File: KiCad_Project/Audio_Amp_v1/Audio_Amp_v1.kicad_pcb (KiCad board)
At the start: 2 copper layers, 93.5 x 52.8 mm, 61 parts, among them IC2 TPA3116D2DAD, IC4 LMR33630ADDA, J1 TS-103-T-A, J2 1729128, J3 1729128, J4 PJ-102AH

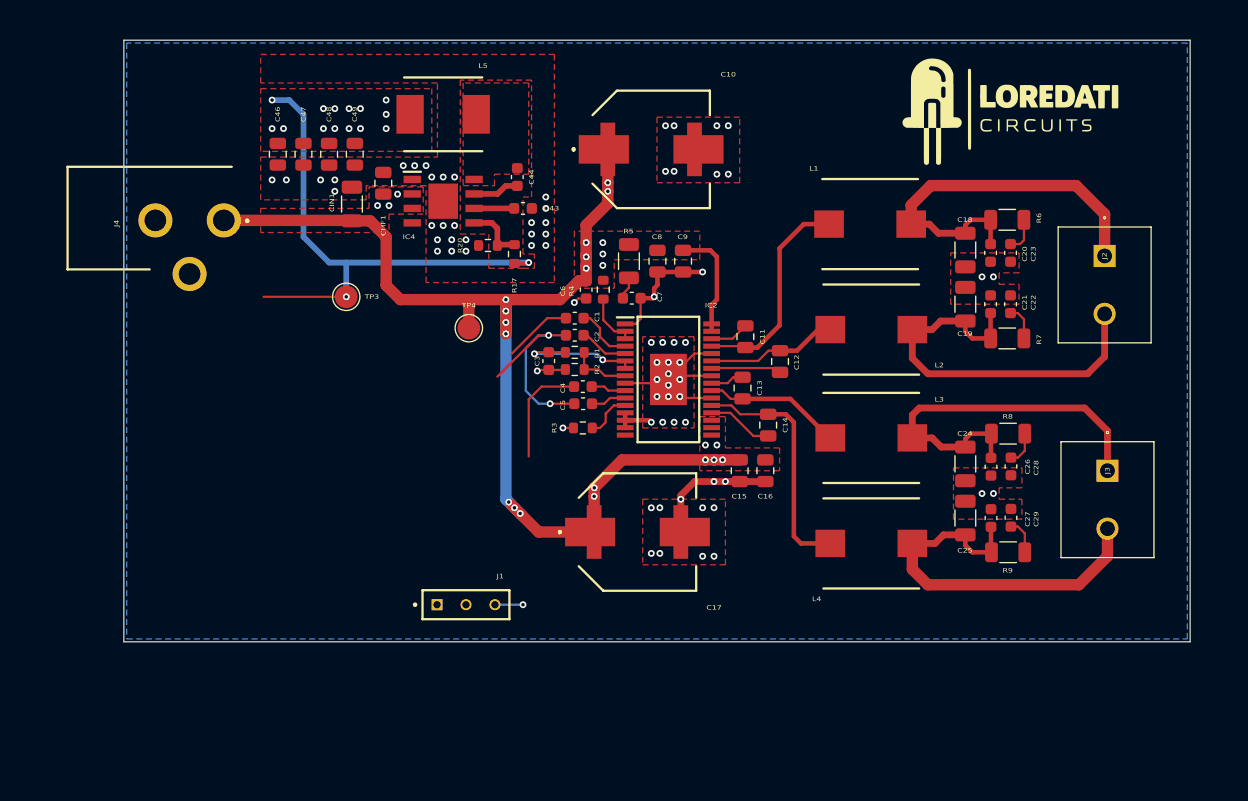
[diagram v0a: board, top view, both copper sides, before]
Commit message: Started routing
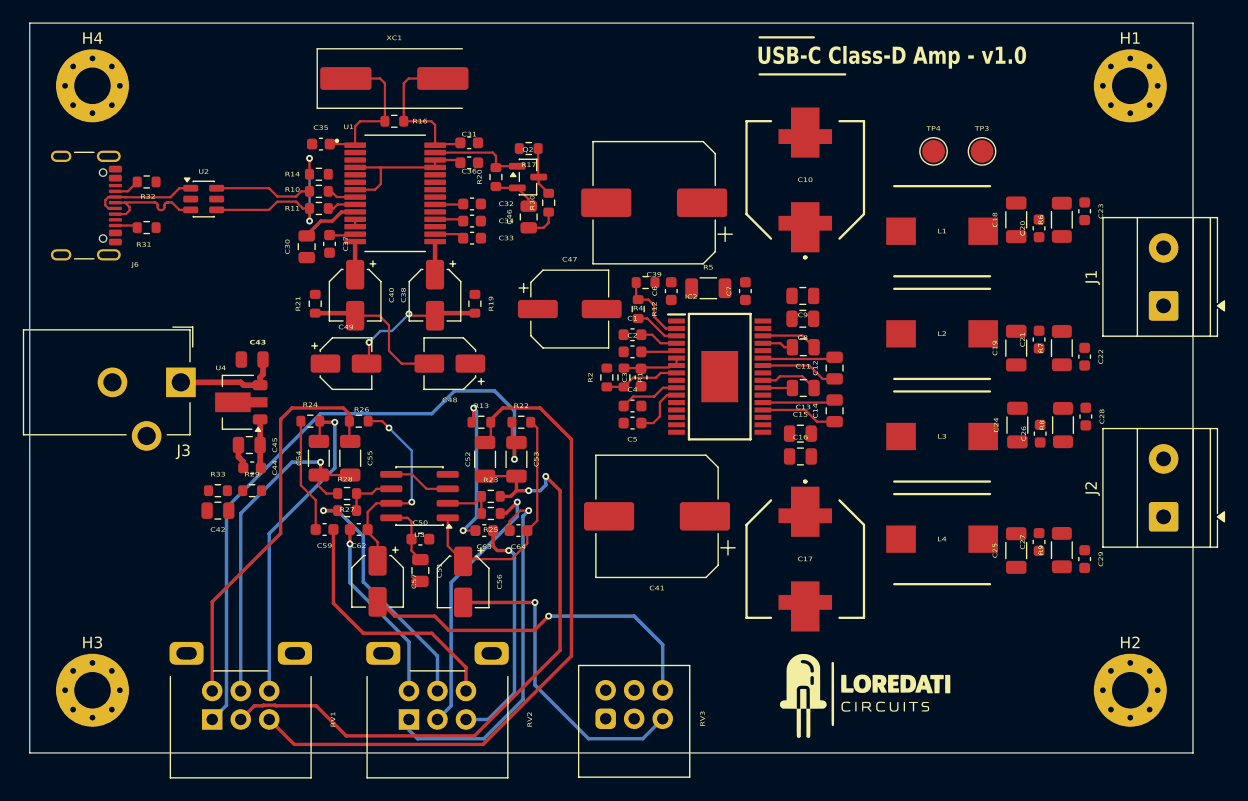
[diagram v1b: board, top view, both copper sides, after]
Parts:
- removed CHF1: 220n, Capacitor_SMD:C_0805_2012Metric
- removed CIN1: 10u, Capacitor_SMD:C_1206_3216Metric
- removed IC4: LMR33630ADDA, LMR33630:SOIC127P600X170-9N
- removed J4: PJ-102AH, 24V-JACK:PJ-102AH
- removed L5: IHLP2525CZER6R8M8A, IHLP2525CZER6R8M8A:INDPM6965X300N
- removed R3: 100k, Resistor_SMD:R_0603_1608Metric
- added C30: 10u, Capacitor_SMD:C_0805_2012Metric, F.Cu at (86.8, 96.9)
- added C31: 1u, Capacitor_SMD:C_0603_1608Metric, F.Cu at (101.0, 89.5)
- added C32: 1u, Capacitor_SMD:C_0603_1608Metric, F.Cu at (101.3, 93.1)
- added C33: 1u, Capacitor_SMD:C_0603_1608Metric, F.Cu at (101.3, 96.1)
- added C34: 10u, Capacitor_SMD:C_0603_1608Metric, F.Cu at (101.3, 94.6)
- added C35: 33p, Capacitor_SMD:C_0603_1608Metric, F.Cu at (88.0, 87.9)
- added C36: 33p, Capacitor_SMD:C_0603_1608Metric, F.Cu at (101.0, 87.8)
- added C37: 1u, Capacitor_SMD:C_0603_1608Metric, F.Cu at (88.8, 96.6)
- added C38: 10u, Capacitor_SMD:CP_Elec_4x5.8, F.Cu at (98.0, 101.1)
- added C39: 470u, Capacitor_SMD:CP_Elec_10x10.5, F.Cu at (117.2, 93.0)
- added C40: 10u, Capacitor_SMD:CP_Elec_4x5.8, F.Cu at (91.0, 101.1)
- added C41: 470u, Capacitor_SMD:CP_Elec_10x10.5, F.Cu at (117.5, 120.5)
- added C42: 10u, Capacitor_SMD:C_0805_2012Metric, F.Cu at (79.0, 120.0)
- added C45: 10u, Capacitor_SMD:C_0805_2012Metric, F.Cu at (81.8, 114.2)
- added C50: 100n, Capacitor_SMD:C_0603_1608Metric, F.Cu at (96.8, 122.5)
- added C51: 10u, Capacitor_SMD:C_0805_2012Metric, F.Cu at (96.8, 125.2)
- added C52: 100n, Capacitor_SMD:C_1206_3216Metric, F.Cu at (102.4, 115.5)
- added C53: 100n, Capacitor_SMD:C_1206_3216Metric, F.Cu at (105.2, 115.5)
- added C54: 100n, Capacitor_SMD:C_1206_3216Metric, F.Cu at (87.8, 115.4)
- added C55: 100n, Capacitor_SMD:C_1206_3216Metric, F.Cu at (90.6, 115.4)
- added C56: 10u, Capacitor_SMD:CP_Elec_4x5.8, F.Cu at (100.5, 126.2)
- added C57: 10u, Capacitor_SMD:CP_Elec_4x5.8, F.Cu at (93.0, 126.2)
- added C59: 2n2, Capacitor_SMD:C_0603_1608Metric, F.Cu at (88.3, 121.7)
- added C62: 2n2, Capacitor_SMD:C_0603_1608Metric, F.Cu at (91.3, 121.7)
- added C63: 2n2, Capacitor_SMD:C_0603_1608Metric, F.Cu at (102.3, 121.8)
- added C64: 2n2, Capacitor_SMD:C_0603_1608Metric, F.Cu at (105.3, 121.8)
- added H1: MountingHole_Pad, MountingHole:MountingHole_3.2mm_M3_Pad_Via, F.Cu at (159.0, 82.8)
- added H2: MountingHole_Pad, MountingHole:MountingHole_3.2mm_M3_Pad_Via, F.Cu at (159.0, 135.8)
- added H3: MountingHole_Pad, MountingHole:MountingHole_3.2mm_M3_Pad_Via, F.Cu at (68.0, 135.8)
- added H4: MountingHole_Pad, MountingHole:MountingHole_3.2mm_M3_Pad_Via, F.Cu at (68.0, 82.8)
- added J6: USB_C_Receptacle_USB2.0_16P, Connector_USB:USB_C_Receptacle_GCT_USB4105-xx-A_16P_TopMnt_Horizontal, F.Cu at (66.3, 93.2)
- added Q2: BSS138, Package_TO_SOT_SMD:SOT-23, F.Cu at (106.2, 90.8)
- added R10: 22, Resistor_SMD:R_0603_1608Metric, F.Cu at (87.9, 92.0)
- added R11: 22, Resistor_SMD:R_0603_1608Metric, F.Cu at (87.9, 93.5)
- added R12: 1k, Resistor_SMD:R_0603_1608Metric, F.Cu at (115.8, 102.3)
- added R13: 10k, Resistor_SMD:R_0603_1608Metric, F.Cu at (102.1, 112.2)
- added R14: 1.5k, Resistor_SMD:R_0603_1608Metric, F.Cu at (87.9, 90.5)
- added R16: 1M, Resistor_SMD:R_0603_1608Metric, F.Cu at (94.5, 85.9)
- added R19: 47k, Resistor_SMD:R_0603_1608Metric, F.Cu at (101.5, 101.9)
- added R21: 47k, Resistor_SMD:R_0603_1608Metric, F.Cu at (87.5, 101.9)
- added R22: 10k, Resistor_SMD:R_0603_1608Metric, F.Cu at (105.6, 112.2)
- added R23: 10k, Resistor_SMD:R_0603_1608Metric, F.Cu at (102.9, 118.8)
- added R24: 10k, Resistor_SMD:R_0603_1608Metric, F.Cu at (87.1, 112.2)
- added R25: 3k3, Resistor_SMD:R_0603_1608Metric, F.Cu at (102.9, 120.2)
- added R26: 10k, Resistor_SMD:R_0603_1608Metric, F.Cu at (91.3, 112.2)
- added R27: 10k, Resistor_SMD:R_0603_1608Metric, F.Cu at (90.3, 118.5)
- added R28: 3k3, Resistor_SMD:R_0603_1608Metric, F.Cu at (90.3, 120.0)
- added R29: 100k, Resistor_SMD:R_0603_1608Metric, F.Cu at (82.0, 118.2)
- added R30: 100k, Resistor_SMD:R_0603_1608Metric, F.Cu at (108.0, 93.0)
- added R31: 5k1, Resistor_SMD:R_0603_1608Metric, F.Cu at (72.8, 95.2)
- added R32: 5k1, Resistor_SMD:R_0603_1608Metric, F.Cu at (72.8, 91.2)
- added R33: 100k, Resistor_SMD:R_0603_1608Metric, F.Cu at (79.0, 118.2)
- added RV1: 100k, Potentiometer_THT:Potentiometer_Alps_RK09L_Double_Horizontal, F.Cu at (78.5, 138.3)
- added RV2: 100k, Potentiometer_THT:Potentiometer_Alps_RK09L_Double_Horizontal, F.Cu at (95.8, 138.3)
- added RV3: 10k, Potentiometer_THT:Potentiometer_Alps_RK097_Dual_Horizontal, F.Cu at (113.0, 138.2)
- added U1: PCM2704CDB, PCM2704CDB:SOP65P780X200-28N, F.Cu at (94.5, 92.2)
- added U2: USBLC6-2SC6, Package_TO_SOT_SMD:SOT-23-6, F.Cu at (77.8, 92.7)
- added U3: OPA1678IDR, Package_SO:SOIC-8_3.9x4.9mm_P1.27mm, F.Cu at (96.7, 118.7)
- added U4: L78L12_SOT89, Package_TO_SOT_SMD:SOT-89-3, F.Cu at (80.8, 110.5)
- added XC1: 12Mhz, Crystal:Crystal_SMD_HC49-SD, F.Cu at (94.5, 82.1)
- C1, C2, C4, C5: value 1u -> 3u3
- C43: value 1u -> 0.33u; footprint Capacitor_SMD:C_0603_1608Metric -> PCM_JLCPCB:C_0805
- C44: value 100n -> 0.1u
- C46: value 22u -> 4u7
- C47: value 22u -> 47u; footprint Capacitor_SMD:C_0805_2012Metric -> Capacitor_SMD:CP_Elec_6.3x5.9
- C48, C49: value 22u -> 10u; footprint Capacitor_SMD:C_0805_2012Metric -> Capacitor_SMD:CP_Elec_4x5.8
- J1: value TS-103-T-A -> Screw_Terminal_01x02; footprint TS_103_T_A:SAMTEC_TS-103-T-A -> TerminalBlock_Phoenix:TerminalBlock_Phoenix_MKDS-1,5-2-5.08_1x02_P5.08mm_Horizontal
- J2: value 1729128 -> Screw_Terminal_01x02; footprint Phoenix-1729128:1729128 -> TerminalBlock_Phoenix:TerminalBlock_Phoenix_MKDS-1,5-2-5.08_1x02_P5.08mm_Horizontal
- J3: value 1729128 -> Barrel_Jack_Switch; footprint Phoenix-1729128:1729128 -> Connector_BarrelJack:BarrelJack_CUI_PJ-102AH_Horizontal
- R17: value 100k -> 47k
- R20: value 43.2k -> 10k
- moved J3 81.6 mm to (75.8, 108.8)
- moved J1 66.5 mm to (161.9, 102.0), turned to 90 degrees
- moved TP3 57.2 mm to (146.0, 88.5)
- moved TP4 43.6 mm to (141.8, 88.5)
- moved C44 34.5 mm to (82.0, 116.2), turned to 180 degrees
- moved C43 27.2 mm to (82.0, 106.8), turned to 180 degrees
- moved C47 27.0 mm to (109.8, 102.3), turned to 0 degrees
- moved J2 23.5 mm to (161.9, 120.5), turned to 90 degrees
- moved C46 22.7 mm to (106.2, 94.2)
- moved C48 21.2 mm to (99.3, 107.1), turned to 180 degrees
- moved C49 18.4 mm to (90.2, 107.1), turned to 0 degrees
- moved C17 14.9 mm to (130.5, 124.2), turned to 180 degrees
- moved C10 13.8 mm to (130.5, 91.0), turned to 0 degrees
- moved C8 13.7 mm to (130.3, 103.2), turned to 180 degrees
- moved C9 10.9 mm to (130.3, 101.2), turned to 180 degrees
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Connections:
- C10 pad 2: IN_COM -> GNDA
- C15 pad 2: IN_COM -> GNDA
- C16 pad 2: IN_COM -> GNDA
- C17 pad 2: IN_COM -> GNDA
- C18 pad 2: IN_COM -> GNDA
- C19 pad 1: IN_COM -> GNDA
- C2 pad 1: IN_COM -> GNDA
- C20 pad 2: IN_COM -> GNDA
- C21 pad 1: IN_COM -> GNDA
- C22 pad 1: IN_COM -> GNDA
- C23 pad 2: IN_COM -> GNDA
- C24 pad 2: IN_COM -> GNDA
- C25 pad 1: IN_COM -> GNDA
- C26 pad 2: IN_COM -> GNDA
- C27 pad 1: IN_COM -> GNDA
- C28 pad 2: IN_COM -> GNDA
- C29 pad 1: IN_COM -> GNDA
- C3 pad 1: IN_COM -> GNDA
- C43 pad 1: Net-(IC4-VCC) -> +24V
- C43 pad 2: IN_COM -> GNDA
- C44 pad 1: Net-(IC4-BOOT) -> +12V
- C44 pad 2: Net-(IC4-SW) -> GNDA
- C46 pad 1: IN_COM -> MUTE
- C46 pad 2: +3.3V -> GNDA
- C47 pad 1: IN_COM -> GNDA
- C47 pad 2: +3.3V -> Net-(IC2-SDZ)
- C48 pad 1: IN_COM -> Net-(C48-Pad1)
- C48 pad 2: +3.3V -> DAC_L
- C49 pad 1: IN_COM -> Net-(C49-Pad1)
- C49 pad 2: +3.3V -> DAC_R
- C5 pad 2: IN_COM -> GNDA
- C6 pad 1: IN_COM -> GNDA
- C7 pad 1: IN_COM -> GNDA
- C8 pad 2: IN_COM -> GNDA
- C9 pad 2: IN_COM -> GNDA
- IC2 pad 1: IN_COM -> GNDA
- IC2 pad 12: Net-(IC2-MUTE) -> MUTE
- IC2 pad 13: IN_COM -> GNDA
- IC2 pad 14: IN_COM -> GNDA
- IC2 pad 15: IN_COM -> GNDA
- IC2 pad 2: Net-(IC2-FAULTZ) -> Net-(IC2-SDZ)
- IC2 pad 22: IN_COM -> GNDA
- IC2 pad 25: IN_COM -> GNDA
- IC2 pad 28: IN_COM -> GNDA
- IC2 pad 33: IN_COM -> GNDA
- IC2 pad 9: IN_COM -> GNDA
- J2 pad 1: OUT_P_RIGHT -> OUT_N_LEFT
- J2 pad 2: OUT_N_RIGHT -> OUT_P_LEFT
- J3 pad 1: OUT_P_LEFT -> +24V
- J3 pad 2: OUT_N_LEFT -> GNDA
- R17 pad 1: Net-(IC4-FB) -> Net-(Q2-D)
- R17 pad 2: +3.3V -> +12V
- R2 pad 2: IN_COM -> GNDA
- R20 pad 1: IN_COM -> GNDA
- R20 pad 2: Net-(IC4-FB) -> /USB_DAC/DAC_ACTIVE
- R4 pad 2: Net-(IC2-FAULTZ) -> Net-(IC2-SDZ)
- TP3 pad 1: +3.3V -> +12V
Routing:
- net +24V: track 107.2 -> 9.41 mm, vias 25 -> 0
- net IN_COM: track 68.1 -> 0.00 mm, vias 79 -> 0
- net Net-(C52-Pad2): track 0.00 -> 60.4 mm
- net Net-(C52-Pad1): track 0.00 -> 57.7 mm, vias 0 -> 2
- net Net-(C53-Pad2): track 0.00 -> 57.0 mm, vias 0 -> 1
- net +3.3V: track 46.2 -> 0.00 mm, vias 16 -> 0
- net Net-(C55-Pad2): track 0.00 -> 35.4 mm
- net OUT_N_RIGHT: track 35.0 -> 0.00 mm
- net OUT_P_RIGHT: track 34.4 -> 0.00 mm
- net OUT_N_LEFT: track 34.0 -> 0.00 mm
- net OUT_P_LEFT: track 34.0 -> 0.00 mm
- net Net-(C64-Pad2): track 0.00 -> 32.3 mm, vias 0 -> 1
- net Net-(C57-Pad2): track 0.00 -> 31.3 mm, vias 0 -> 1
- net Net-(C54-Pad1): track 0.00 -> 31.3 mm, vias 0 -> 1
- net Net-(C54-Pad2): track 0.00 -> 29.1 mm, vias 0 -> 1
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- removed copper zone on F.Cu, net +24V
- removed copper zone on F.Cu, net +3.3V
- removed copper zone on B.Cu, net IN_COM
- removed copper zone on F.Cu, net IN_COM
- removed copper zone on F.Cu, net Net-(IC4-SW)
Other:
- board size 93.5 x 52.8 mm -> 102 x 64 mm
- copper layers 2 -> 4
- board text added: "USB-C Class-D Amp - v1.0"
